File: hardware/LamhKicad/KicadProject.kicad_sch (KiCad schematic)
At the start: 50 parts, among them J1 JTAG-10 PIN, J2 436500303, J3 436500303, J4 436500303, J5 ESQ-110-X-X-D, J6 436500303, U1 TJA1051T-3, U2 PCA9685PW_112, U3 TLV70433DBVT, U4 STM32F072C8Tx

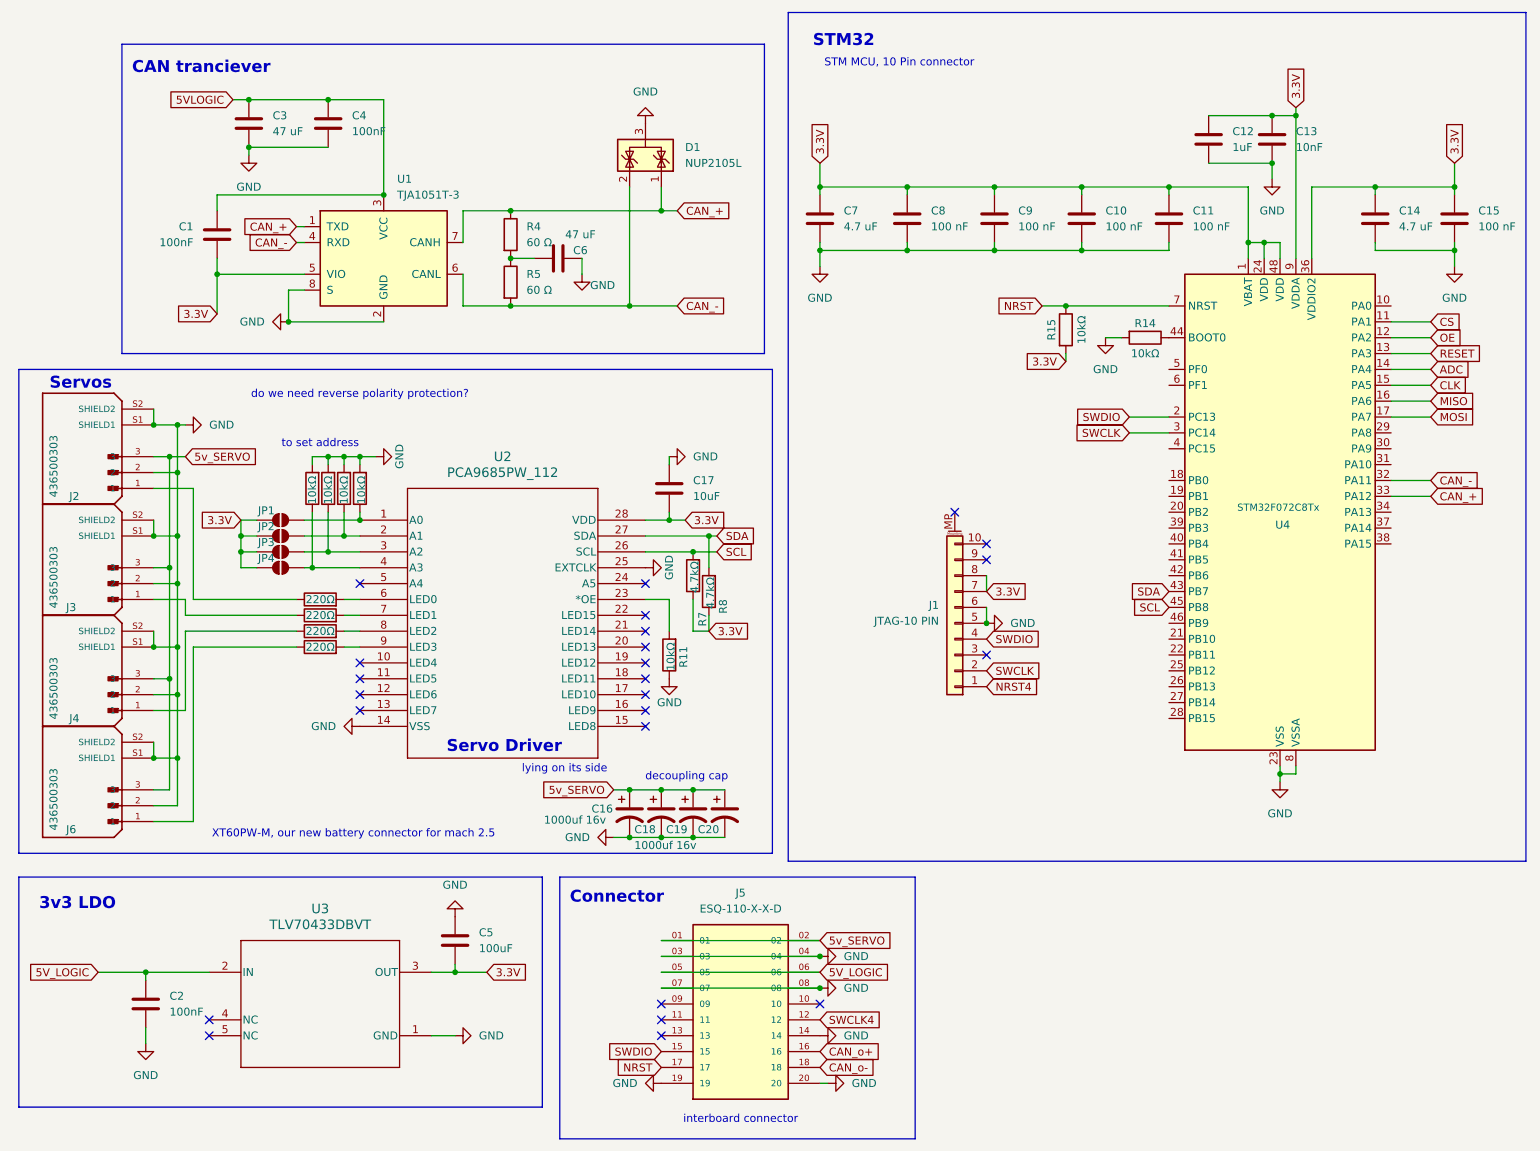
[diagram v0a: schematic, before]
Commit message: minor changes
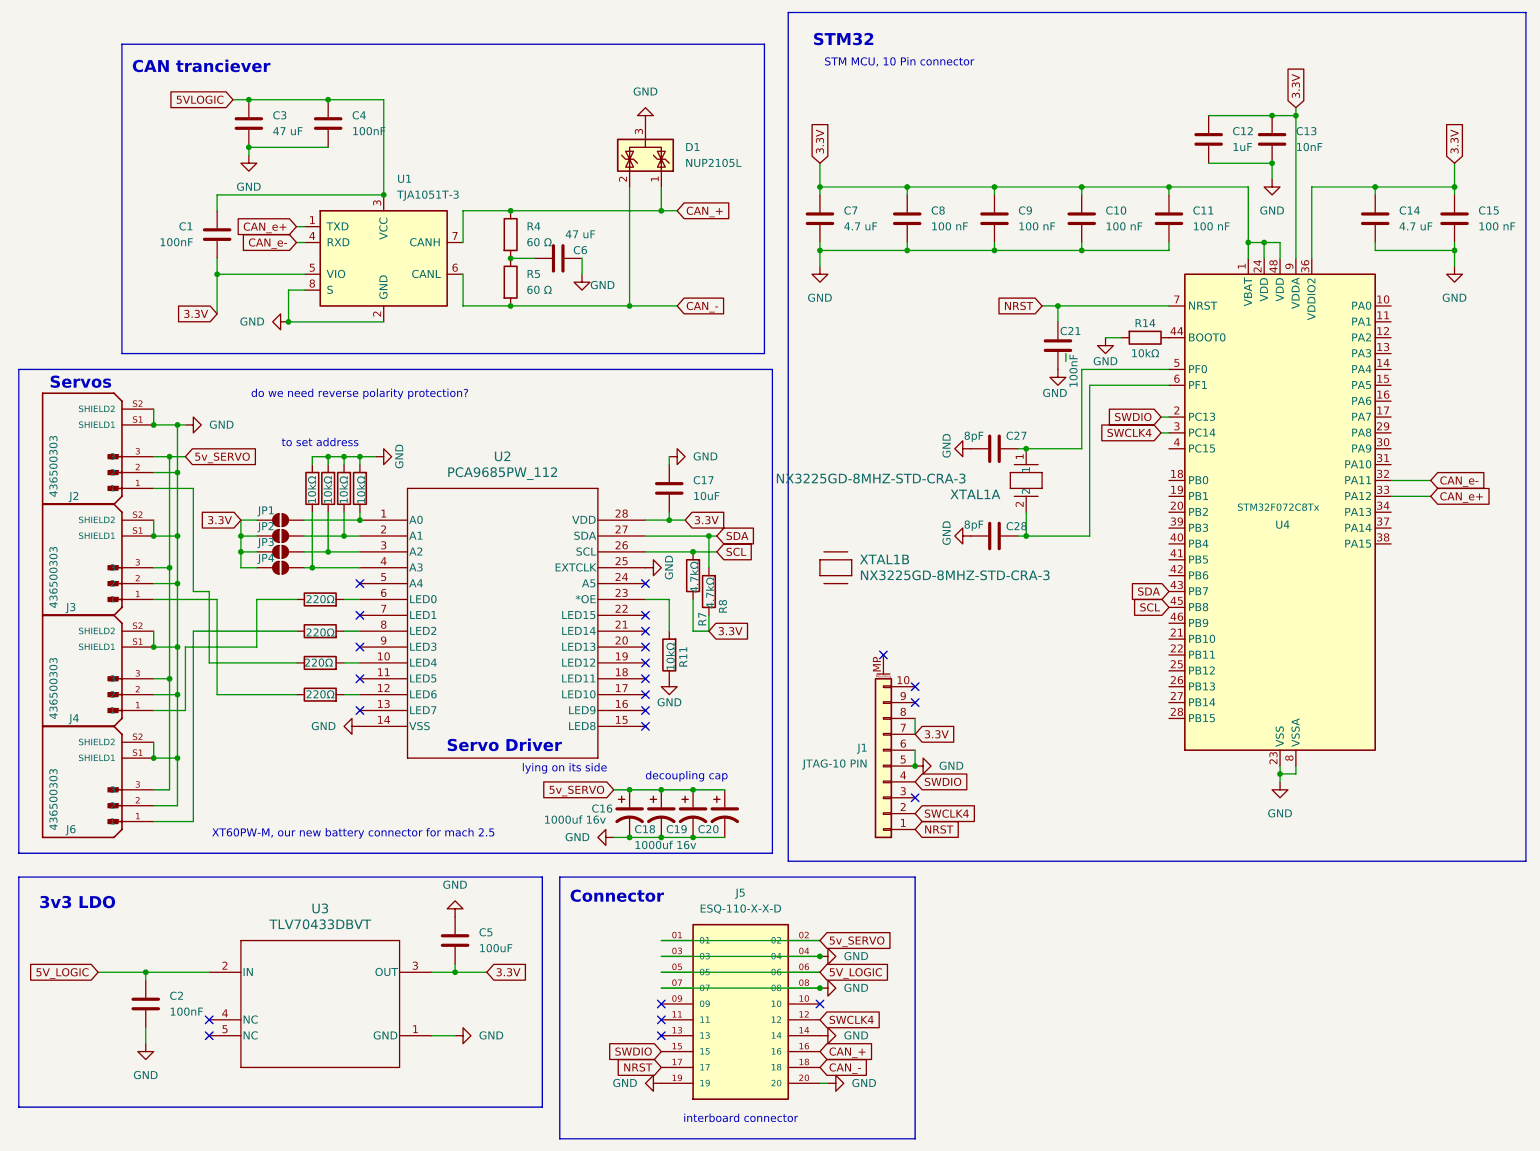
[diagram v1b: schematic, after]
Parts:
- removed R15: 10kΩ, Resistor_SMD:R_0402_1005Metric, symbol Device:R
- added C21: 100nF, Capacitor_SMD:C_0402_1005Metric, symbol Device:C
- added C27, C28: 8pF, Capacitor_SMD:C_0402_1005Metric, symbol Device:C
- added XTAL1: NX3225GD-8MHZ-STD-CRA-3, XTAL_NX3225GD-8MHZ-STD-CRA-3_NDK, symbol STDCRA38M:NX3225GD-8MHZ-STD-CRA-3
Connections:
- net CAN_o+ is gone; now on net CAN_+: J5.16
- net CAN_o- is gone; now on net CAN_-: J5.18
- net NRST4 is gone; now on net NRST: J1.1 (Pin_1)
- net SWCLK is gone; now on net SWCLK4: J1.2 (Pin_2), U4.3 (PC14)
- net CAN_+: no longer U1.1 (TXD), U4.33 (PA12)
- net CAN_-: no longer U1.4 (RXD), U4.32 (PA11)
- net GND: now also C21.2, C27.1, C28.2
- net NRST: now also C21.1
- net at R3.1: now also J2.1; no longer J4.1
- net at R3.2: now also U2.10 (LED4); no longer U2.8 (LED2)
- net at U4.5 (PF0): now also C27.2, XTAL1.1
- net at U4.6 (PF1): now also C28.1, XTAL1.2
- net at U2.12 (LED6): now also R6.2
- net at U2.7 (LED1): no longer R2.2
- net at U2.9 (LED3): no longer R6.2
- net at R1.1: now also J4.1; no longer J2.1
- net at J3.1: now also R6.1; no longer R2.1
- net at J6.1: now also R2.1; no longer R6.1
- net ADC: no longer names the net of U4.14 (PA4)
- net CLK: no longer names the net of U4.15 (PA5)
- net CS: no longer names the net of U4.11 (PA1)
- net MISO: no longer names the net of U4.16 (PA6)
- net MOSI: no longer names the net of U4.17 (PA7)
- net OE: no longer names the net of U4.12 (PA2)
- net RESET: no longer names the net of U4.13 (PA3)
- new net: R2.2, U2.8 (LED2)
- new net CAN_e+: U1.1 (TXD), U4.33 (PA12)
- new net CAN_e-: U1.4 (RXD), U4.32 (PA11)
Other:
- moved on the sheet: J1
